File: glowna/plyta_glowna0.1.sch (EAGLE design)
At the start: 119 parts, among them IC1 4504D, Q1 CSM-7X-DU, Q2 N-HEXFET-2D_SOT232-IRLL014N, Q3 N-HEXFET-2D_SOT232-IRLL014N, Q4 N-HEXFET-2D_SOT232-IRLL014N, Q5 N-HEXFET-2D_SOT232-IRLL014N, Q6 N-HEXFET-2D_SOT232-IRLL014N, X1 MINI-USB_SHIELD5P2-32005-601

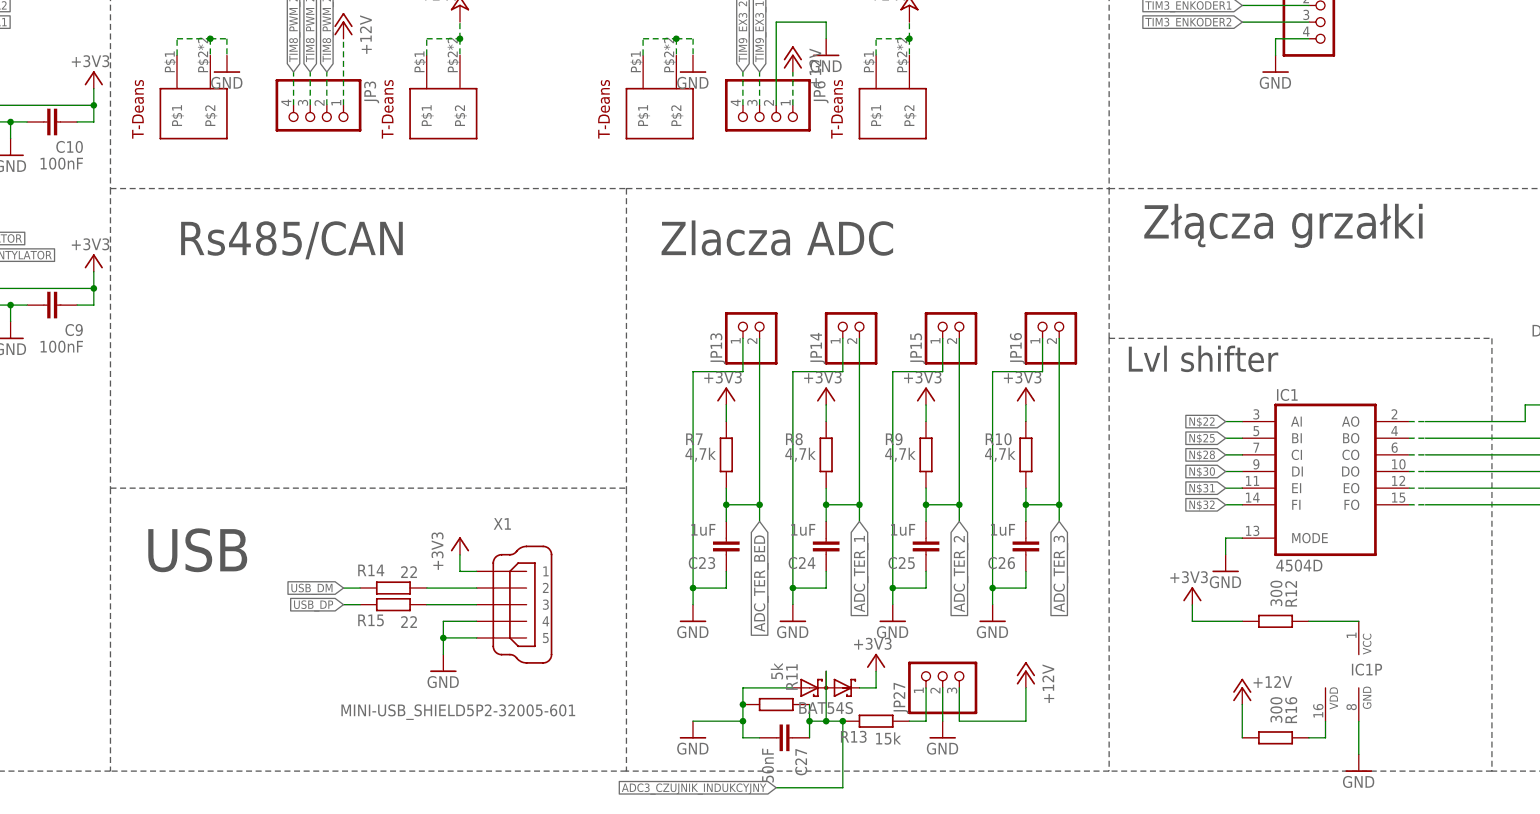
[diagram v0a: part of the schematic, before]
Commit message: rs i termistory
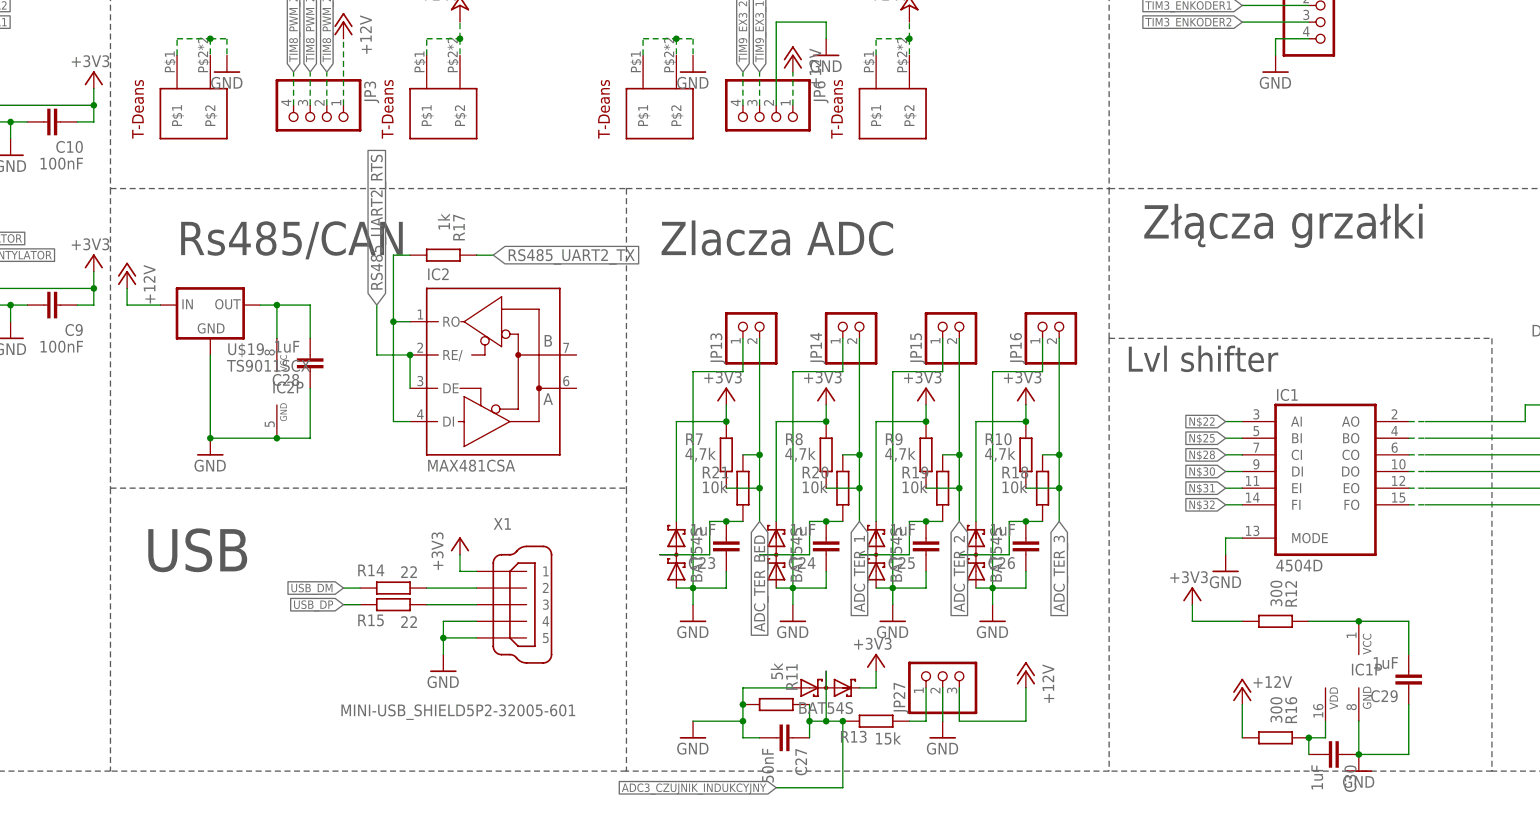
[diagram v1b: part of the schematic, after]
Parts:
- added C28, C29, C30: 1uF, rcl:C-EUC0603
- added D1, D2, D3, D4: BAT54S, diode:BAT54S
- added IC2: MAX481CSA, maxim:MAX481CSA
- added R17: 1k, rcl:R-EU_R0603
- added R18, R19, R20, R21: 10k, rcl:R-EU_R0603
- added U$19: TS9011SCX, v-reg:TS9011SCX
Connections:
- new net N$40: C28.2, IC2P.VCC, U$19.OUT
- new net N$42: C25.2, D3.C1A2, R19.2
- new net N$43: C24.2, D2.C1A2, R20.2
- new net N$44: C26.2, D4.C1A2, R18.2
- new net N$47: C23.2, D1.C1A2, R21.2
- net +12V: now also U$19.IN
- net +3V3: now also D1.C2, D2.C2, D3.C2, D4.C2
- net ADC_TER_1: now also R20.1; no longer C24.2
- net ADC_TER_2: now also R19.1; no longer C25.2
- net ADC_TER_3: now also R18.1; no longer C26.2
- net ADC_TER_BED: now also R21.1; no longer C23.2
- net GND: now also C28.1, C29.1, C30.1, D1.A1, D2.A1, D3.A1, D4.A1, IC2P.GND, U$19.GND
- net N$16: now also C29.2
- net N$39: now also C30.2
- net RS485_UART2_RTS: now also IC2G$1.DE, IC2G$1.RE/
- net RS485_UART2_TX: now also IC2G$1.DI, IC2G$1.RO, R17.1, R17.2
